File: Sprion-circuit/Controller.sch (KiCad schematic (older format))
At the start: 22 parts, among them J2 Conn_01x04_Female, Q3 Q_NMOS_GSD, Q4 Q_NMOS_GSD, SW2 SW_Push, SW3 SW_Push, SW4 SW_Push, U3 STM32F405RGTx

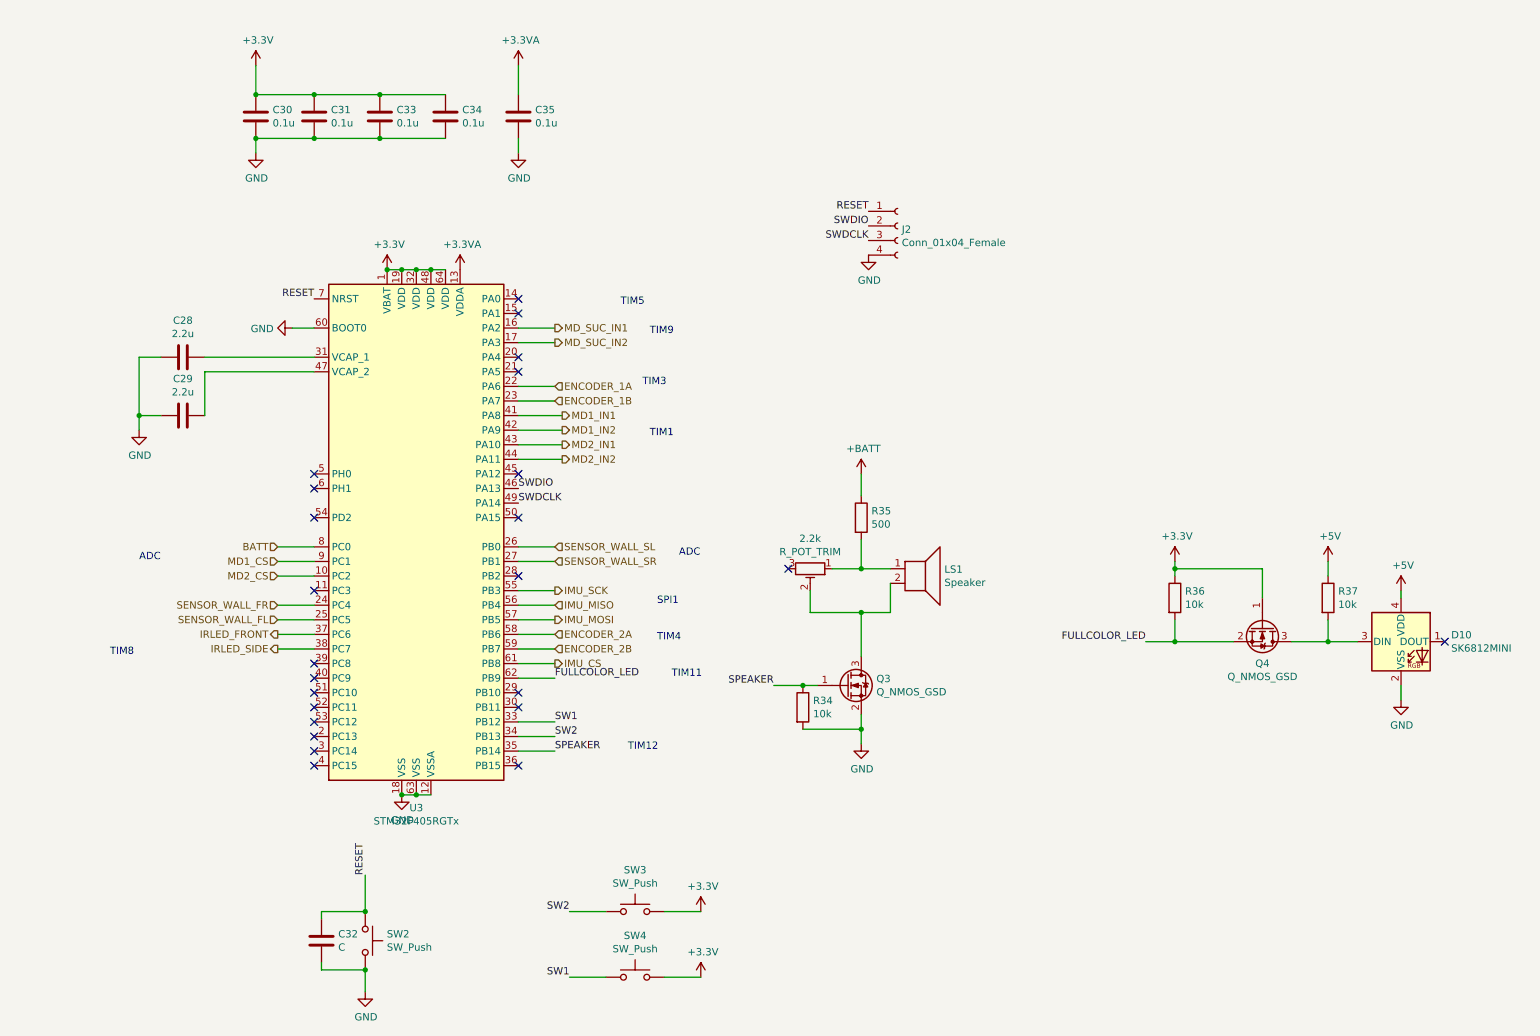
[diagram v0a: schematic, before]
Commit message: add,feat,fix:すまんコミットわすれててぐちゃぐちゃや
配置始めた。
フットプリント割り当てた
回路図pdfで吐いた
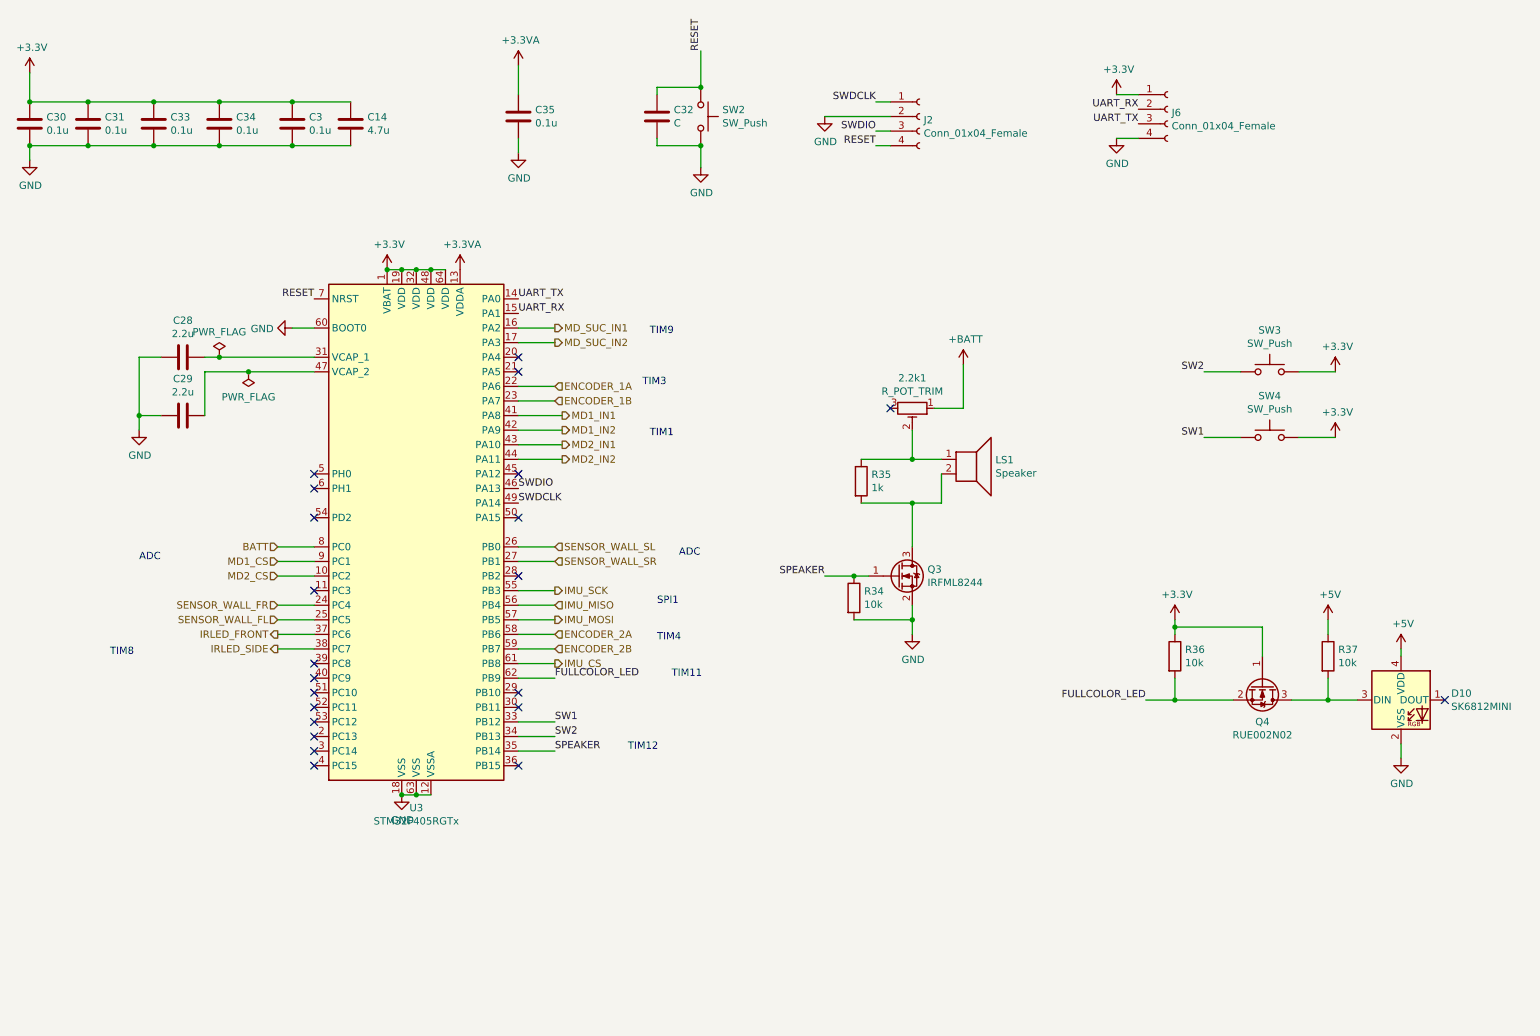
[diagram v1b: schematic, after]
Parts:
- added C14: 4.7u, Capacitor_SMD:C_0603_1608Metric, symbol Device:C
- added C3: 0.1u, Capacitor_SMD:C_0603_1608Metric, symbol Device:C
- added J6: Conn_01x04_Female, Connector_JST:JST_SH_SM04B-SRSS-TB_1x04-1MP_P1.00mm_Horizontal, symbol Connector:Conn_01x04_Female
- 2.2k1: renamed from 2.2k; footprint (none) -> Sprion-circuit:Potentiometer_SMD_PVZ3A
- C28, C29, C30, C31, C32, C33, C34, C35: footprint (none) -> Capacitor_SMD:C_0603_1608Metric
- J2: footprint (none) -> Connector_JST:JST_SH_SM04B-SRSS-TB_1x04-1MP_P1.00mm_Horizontal
- LS1: footprint (none) -> Sprion-circuit:PKMCS
- Q3: value Q_NMOS_GSD -> IRFML8244; footprint (none) -> Package_TO_SOT_SMD:SOT-23
- Q4: value Q_NMOS_GSD -> RUE002N02; footprint (none) -> Package_TO_SOT_SMD:SOT-416
- R34, R36, R37: footprint (none) -> Resistor_SMD:R_0603_1608Metric
- R35: value 500 -> 1k; footprint (none) -> Resistor_SMD:R_0603_1608Metric
- SW2, SW3, SW4: footprint (none) -> Sprion-circuit:SMT_4.2X3.2_
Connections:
- net +3V3: now also C14.1, C3.1, J6.1 (Pin_1)
- net +BATT: now also 2.2k1.1; no longer R35.1
- net GND: now also J2.2 (Pin_2), C14.2, C3.2, J6.4 (Pin_4); no longer J2.4 (Pin_4)
- net RESET: now also J2.4 (Pin_4); no longer J2.1 (Pin_1)
- net SWDCLK: now also J2.1 (Pin_1); no longer J2.3 (Pin_3)
- net SWDIO: now also J2.3 (Pin_3); no longer J2.2 (Pin_2)
- net UART_TX: now reaches U3.14 (PA0)
- net UART_TX: now also J6.3 (Pin_3)
- net UART_RX: now reaches U3.15 (PA1)
- net UART_RX: now also J6.2 (Pin_2)
- net at LS1.2, Q3.3 (D): now also R35.2; no longer 2.2k1.2
- new net: 2.2k1.2, LS1.1, R35.1
- no-connect marks 24 -> 22
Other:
- note removed: "TIM5\n"
- moved on the sheet: 2.2k1, C30, C31, C32, C33, C34, D10, J2, LS1, Q3, Q4, R34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
